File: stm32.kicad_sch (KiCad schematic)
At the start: 43 parts, among them J1 TC2030, J2 USB_C_Receptacle_PowerOnly_6P, SW1 SW_Push, U1 STM32F411CEUx, U2 BMI088, U3 BMP388, U4 W25Q128JVSIQ, U5 TP4056-42-ESOP8, Y1 Crystal_GND24

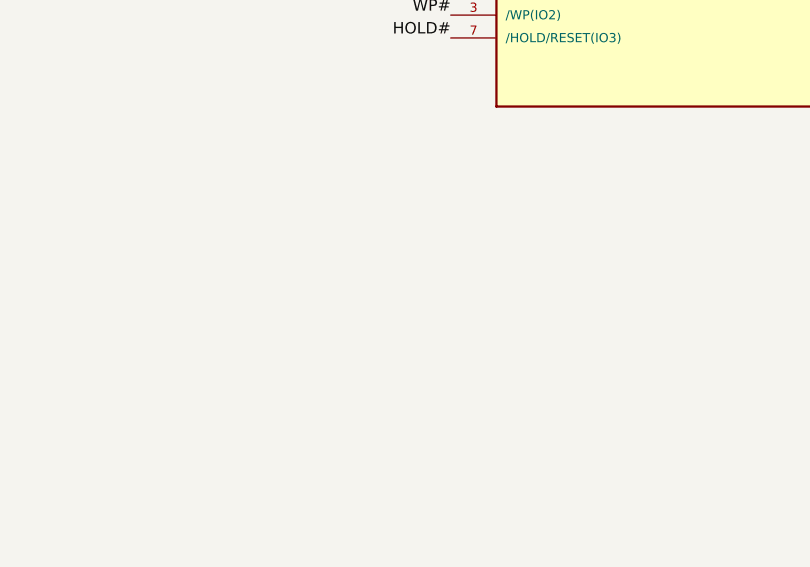
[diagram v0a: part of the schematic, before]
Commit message: small update
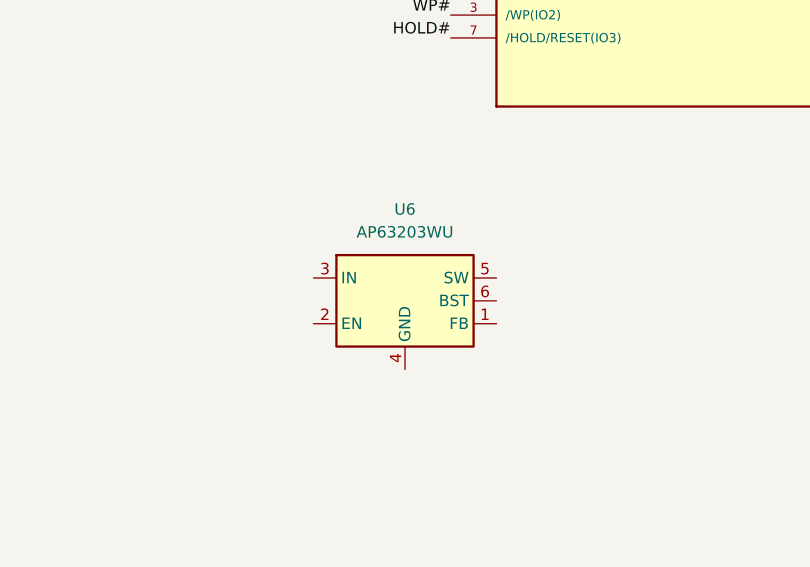
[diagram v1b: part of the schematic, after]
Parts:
- added U6: AP63203WU, Package_TO_SOT_SMD:TSOT-23-6, symbol Regulator_Switching:AP63203WU
- R10, R11, R12, R23, R24, R9: footprint 240Library:STA_CF14_STP -> Resistor_SMD:R_0402_1005Metric
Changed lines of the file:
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@@
 	)
 	(symbol
+		(lib_id "Regulator_Switching:AP63203WU")
+		(at 180.34 123.19 0)
+		(unit 1)
+		(exclude_from_sim no)
+		(in_bom yes)
+		(on_board yes)
+		(dnp no)
+		(fields_autoplaced yes)
+		(property "Reference" "U6"
+			(at 180.34 113.03 0)
+			(effects
+				(font
+					(size 1.27 1.27)
+				)
+			)
+		)
+		(property "Value" "AP63203WU"
+			(at 180.34 115.57 0)
+			(effects
+				(font
+					(size 1.27 1.27)
+				)
+			)
+		)
+		(property "Footprint" "Package_TO_SOT_SMD:TSOT-23-6"
+			(at 180.34 146.05 0)
+			(effects
+				(font
+					(size 1.27 1.27)
+				)
+				(hide yes)
+			)
+		)
+		(property "Datasheet" "https://www.diodes.com/assets/Datasheets/AP63200-AP63201-AP63203-AP63205.pdf"
+			(at 180.34 123.19 0)
+			(effects
+				(font
+					(size 1.27 1.27)
+				)
+				(hide yes)
+			)
+		)
+		(property "Description" "2A, 1.1MHz Buck DC/DC Converter, fixed 3.3V output voltage, TSOT-23-6"
+			(at 180.34 123.19 0)
+			(effects
+				(font
+					(size 1.27 1.27)
+				)
+				(hide yes)
+			)
+		)
+		(pin "1"
+		)
+		(pin "6"
+		)
+		(pin "5"
+		)
+		(pin "4"
+		)
+		(pin "2"
+		)
+		(pin "3"
+		)
+		(instances
+			(project ""
+				(path "/807257e6-524f-404b-b91f-049b9c2bdd5b"
+					(reference "U6")
+					(unit 1)
+				)
+			)
+		)
+	)
+	(symbol
 		(lib_id "power:+5V")
 		(at 46.99 161.29 0)
@@
 			)
 		)
-		(property "Footprint" "240Library:STA_CF14_STP"
+		(property "Footprint" "Resistor_SMD:R_0402_1005Metric"
 			(at 130.81 162.56 0)
 			(effects
@@
 			)
 		)
-		(property "Footprint" "240Library:STA_CF14_STP"
+		(property "Footprint" "Resistor_SMD:R_0402_1005Metric"
 			(at 118.11 177.8 0)
 			(effects
@@
 			)
 		)
-		(property "Footprint" "240Library:STA_CF14_STP"
+		(property "Footprint" "Resistor_SMD:R_0402_1005Metric"
 			(at 97.79 162.56 0)
 			(effects
@@
 			)
 		)
-		(property "Footprint" "240Library:STA_CF14_STP"
+		(property "Footprint" "Resistor_SMD:R_0402_1005Metric"
 			(at 71.12 165.1 0)
 			(effects
@@
 			)
 		)
-		(property "Footprint" "240Library:STA_CF14_STP"
+		(property "Footprint" "Resistor_SMD:R_0402_1005Metric"
 			(at 97.79 165.1 0)
 			(effects
@@
 			)
 		)
-		(property "Footprint" "240Library:STA_CF14_STP"
+		(property "Footprint" "Resistor_SMD:R_0402_1005Metric"
 			(at 71.12 176.53 0)
 			(effects

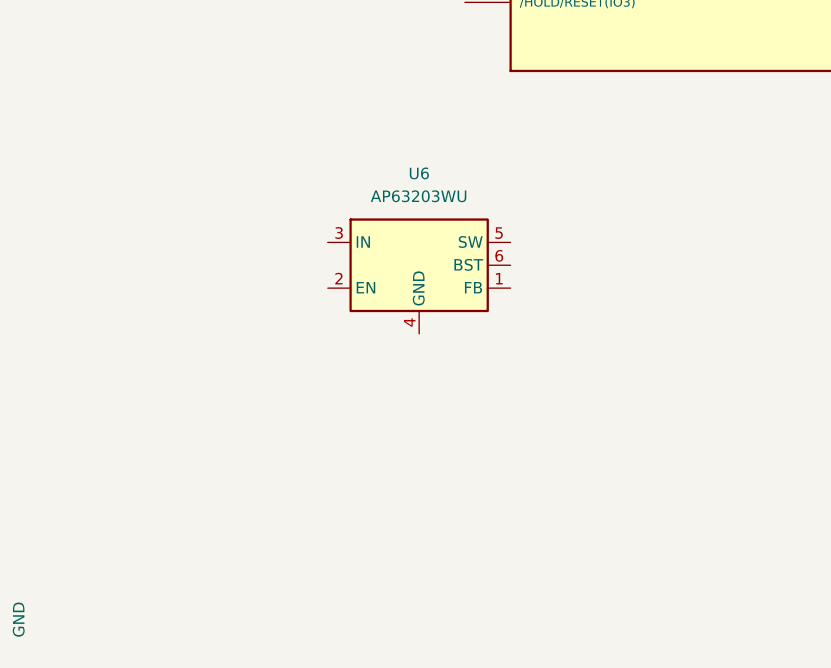
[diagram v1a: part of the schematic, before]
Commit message: replaced buck
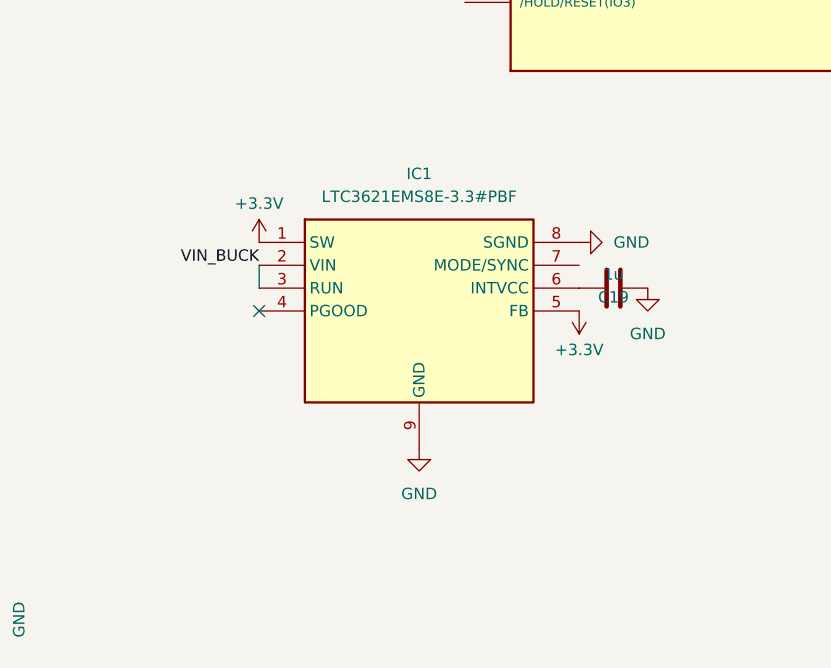
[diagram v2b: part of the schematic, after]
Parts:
- removed U6: AP63203WU, Package_TO_SOT_SMD:TSOT-23-6, symbol Regulator_Switching:AP63203WU
- added C19: 1u, Capacitor_SMD:C_0402_1005Metric, symbol Device:C
- added IC1: LTC3621EMS8E-3.3#PBF, SOP65P490X110-9N, symbol 2026-04-12_18-39-20:LTC3621EMS8E-3.3#PBF
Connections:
- net +3.3V: now also IC1.1 (SW), IC1.5 (FB)
- net GND: now also C19.1, IC1.8 (SGND), IC1.9 (GND)
- new net: C19.2, IC1.6 (INTVCC)
- new net VIN_BUCK: IC1.2 (VIN), IC1.3 (RUN)
- no-connect marks 3 -> 4
